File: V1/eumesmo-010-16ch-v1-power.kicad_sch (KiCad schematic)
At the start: 51 parts, among them J6 250-202, J7 USB_C_Receptacle_USB2.0, Q1 WPM2015-3/TR, Q2 MMUN2211LT3G, U1 TX4138, U2 SY8089A1AAC

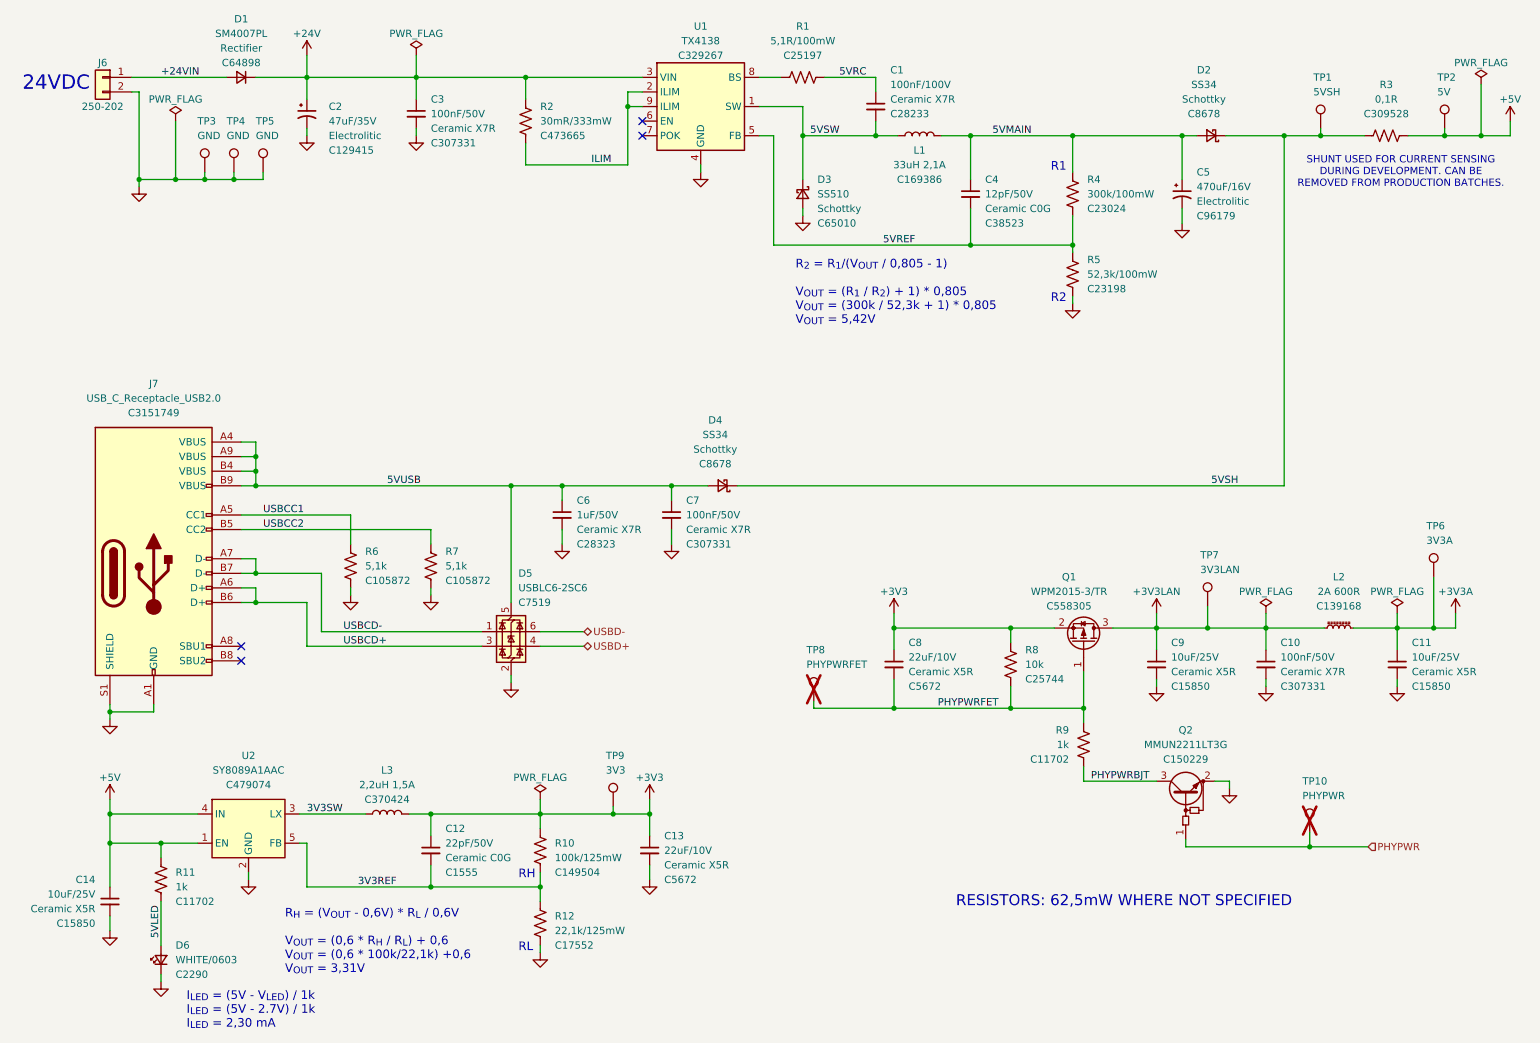
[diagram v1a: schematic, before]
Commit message: Restarting fresh
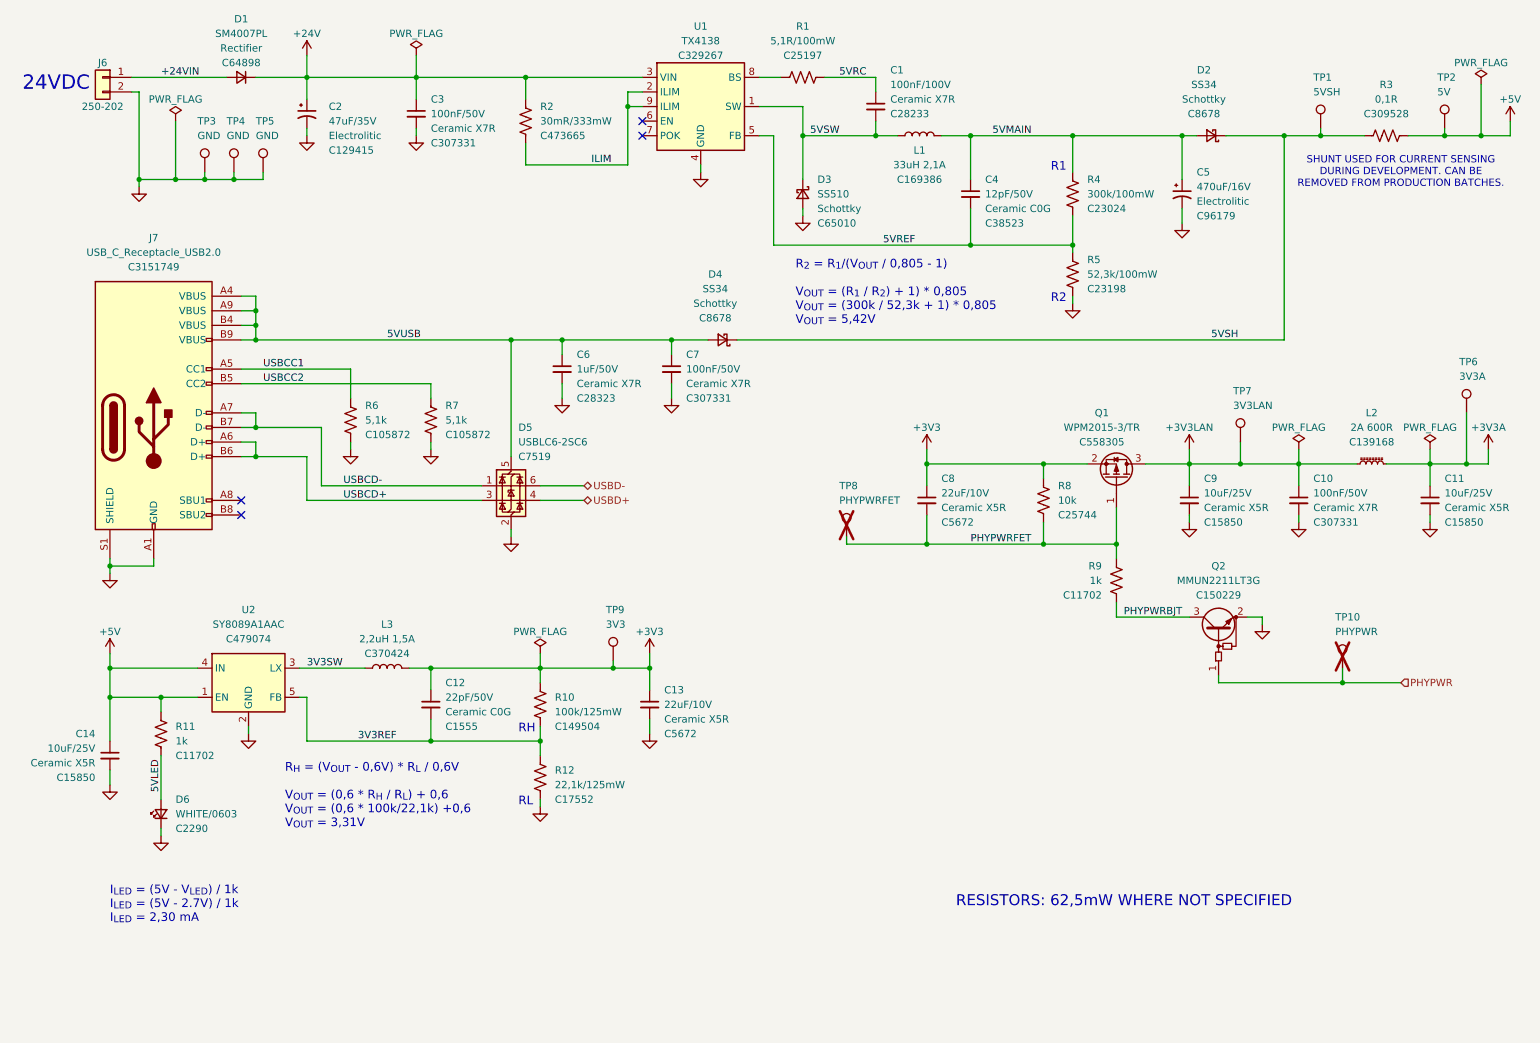
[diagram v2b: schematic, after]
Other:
- moved on the sheet: C10, C11, C12, C13, C14, C6, C7, C8, C9, D4, D5, D6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
